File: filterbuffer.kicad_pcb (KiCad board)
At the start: 2 copper layers, 128.5 x 38 mm, 27 parts, among them J1 Conn_01x02, J10 Conn_01x02, J11 Conn_01x02, J12 Conn_01x02, J13 Conn_01x02, J14 Conn_01x02, J15 Conn_01x02, J16 Conn_01x02, J2 Conn_01x02, J3 Conn_01x02, J4 Conn_01x02, J5 Conn_01x02, J6 Conn_01x02, J7 Conn_01x02, J8 Conn_01x02, J9 Conn_01x02

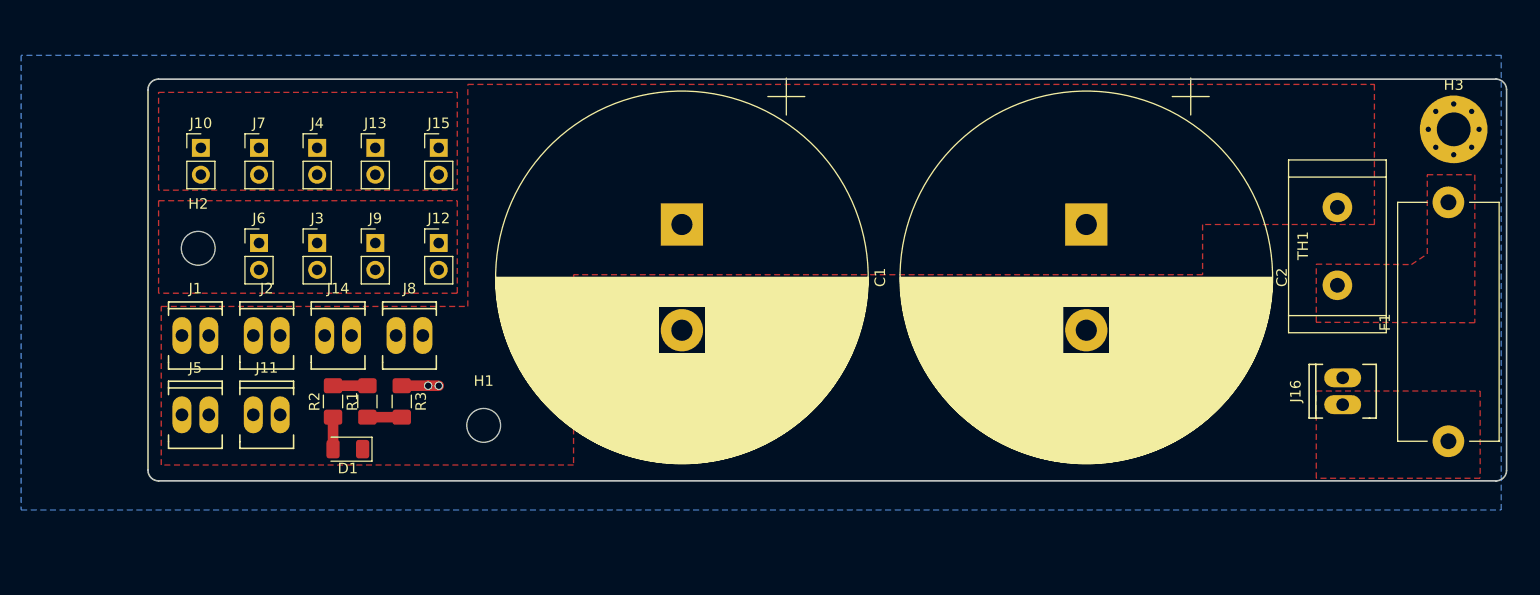
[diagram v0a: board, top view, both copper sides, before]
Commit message: update layout
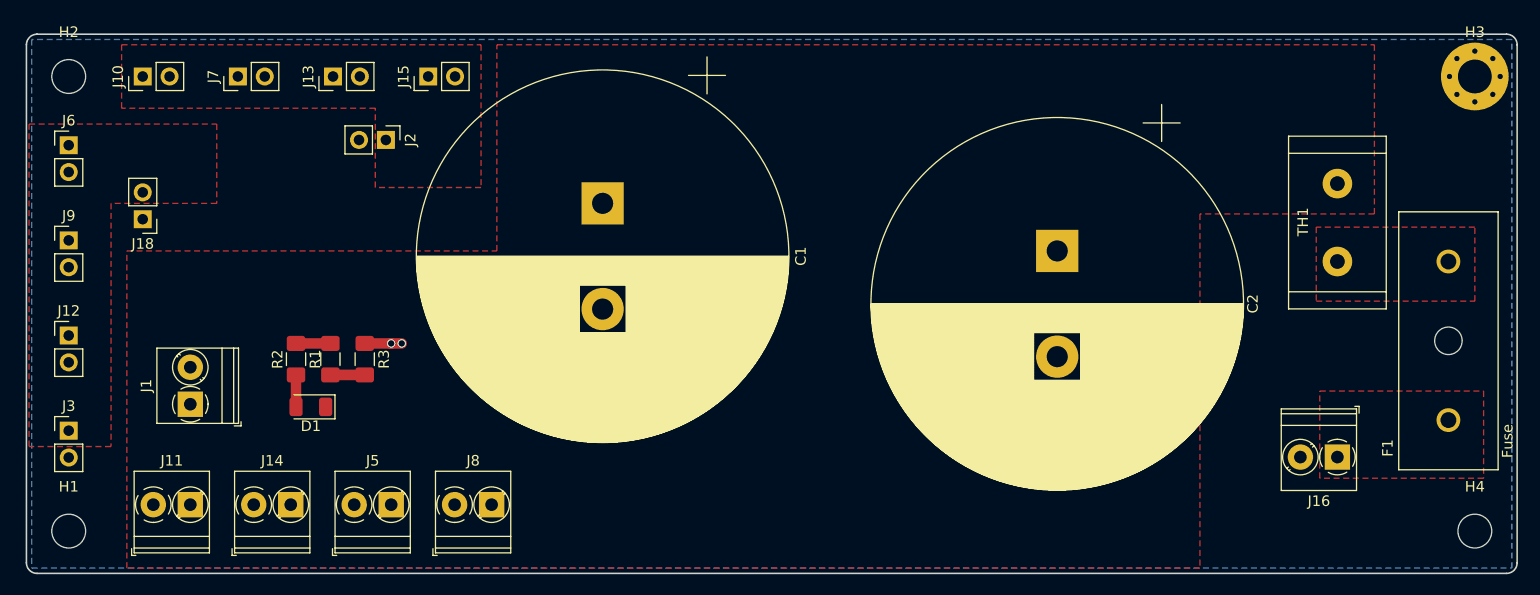
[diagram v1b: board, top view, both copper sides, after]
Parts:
- removed J4: Conn_01x02, Connector_PinHeader_2.54mm:PinHeader_1x02_P2.54mm_Vertical
- added H4: MountingHole, MountingHole:MountingHole_3.2mm_M3, F.Cu at (182.7, 142.2)
- added J18: Conn_01x02, Connector_PinHeader_2.54mm:PinHeader_1x02_P2.54mm_Vertical, F.Cu at (56.7, 112.7)
- F1: footprint Fuse:Fuseholder_Cylinder-5x20mm_Stelvio-Kontek_PTF78_Horizontal_Open -> 696105003002:FUSE_696105003002
- J1, J11, J14, J16, J5, J8: footprint Sockets_MOLEX_KK-System:Socket_MOLEX-KK-RM2-54mm_Lock_2pin_straight -> TerminalBlock_Phoenix:TerminalBlock_Phoenix_PT-1,5-2-3.5-H_1x02_P3.50mm_Horizontal
- J2: footprint Sockets_MOLEX_KK-System:Socket_MOLEX-KK-RM2-54mm_Lock_2pin_straight -> Connector_PinHeader_2.54mm:PinHeader_1x02_P2.54mm_Vertical
- moved H1 40.5 mm to (49.7, 142.2)
- moved J12 36.1 mm to (49.7, 123.7)
- moved J3 29.5 mm to (49.7, 132.7)
- moved J9 29.0 mm to (49.7, 114.7)
- moved J2 21.7 mm to (79.7, 105.2), turned to 270 degrees
- moved H2 20.4 mm to (49.7, 99.2)
- moved J6 20.2 mm to (49.7, 105.7)
- moved J14 17.9 mm to (67.2, 139.7)
- moved J5 17.3 mm to (76.7, 139.7)
- moved J8 16.6 mm to (86.2, 139.7)
- moved J11 13.7 mm to (57.7, 139.7)
- moved F1 9.50 mm to (180.2, 124.2)
- moved J10 8.71 mm to (56.7, 99.2), turned to 90 degrees
- moved J13 7.85 mm to (74.7, 99.2), turned to 90 degrees
- moved C1 7.76 mm to (100.2, 111.2)
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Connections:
- H3 pad 1: Net-(H3-Pad1) -> GND
- J2 pad 1: VCC -> +5V
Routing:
- added copper zone on F.Cu, net (none)
- removed copper zone on F.Cu, net Net-(F1-Pad2)
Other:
- board size 128.5 x 38 mm -> 141 x 51 mm
